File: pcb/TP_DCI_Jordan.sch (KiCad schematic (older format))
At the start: 19 parts, among them J1 MICRO, J2 Display, SW1 SW_DIP_x03, U1 PCF8574

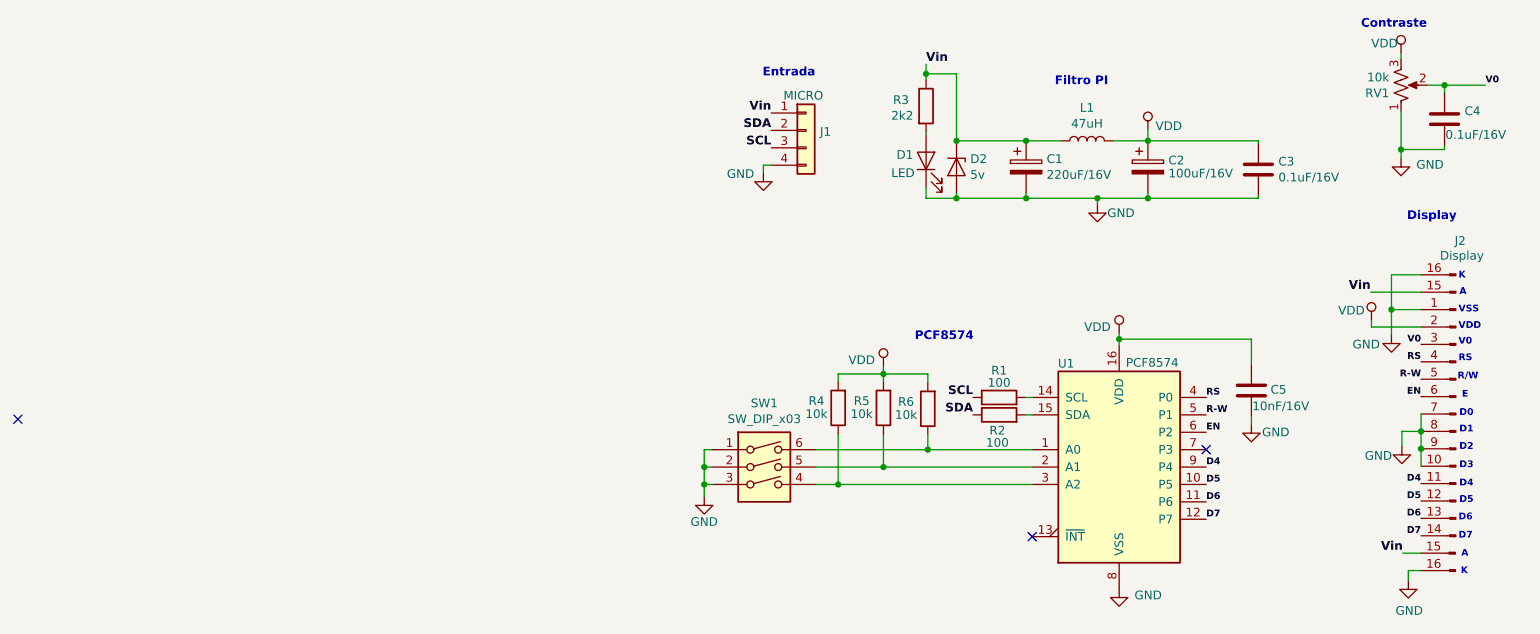
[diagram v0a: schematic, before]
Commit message: mejora de esquemático
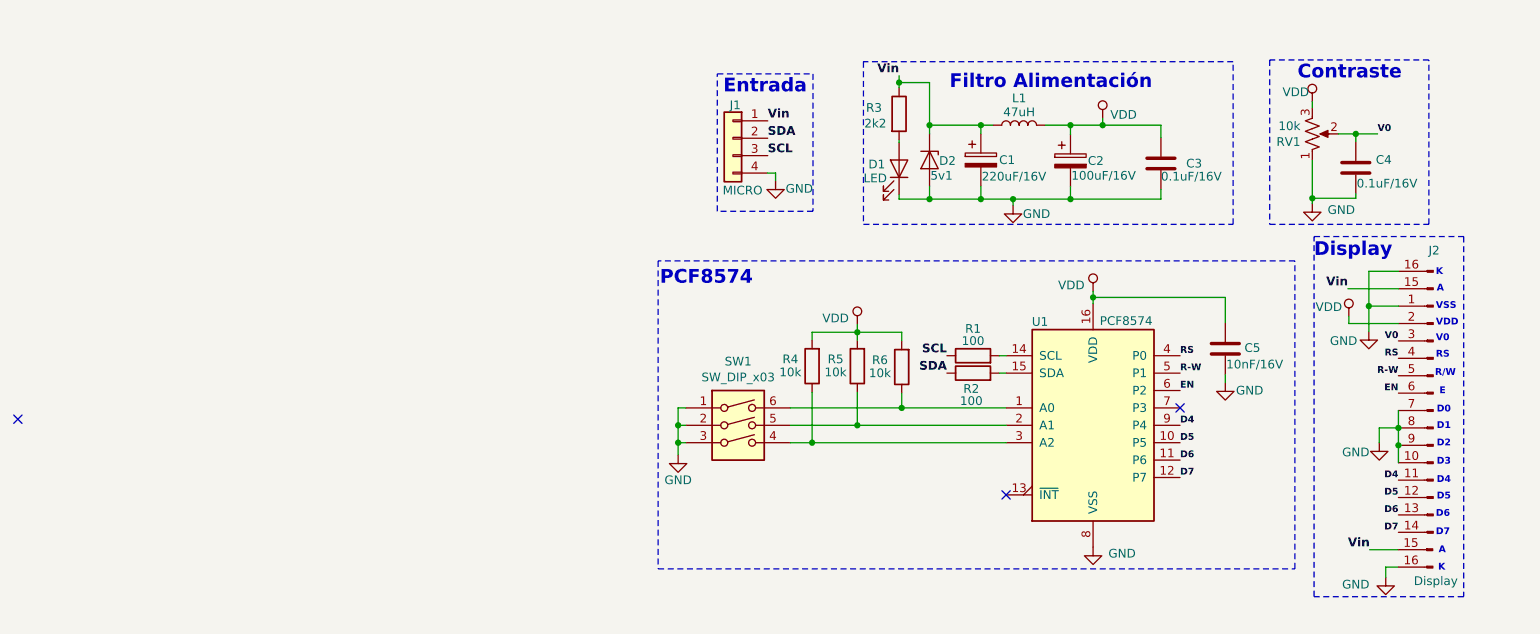
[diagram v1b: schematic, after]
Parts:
- C3, C4, C5: footprint miCapacitor_THT:Lenteja_Ceramica -> Capacitor_SMD:C_0805_2012Metric
- D2: value 5v -> 5v1
- R1, R2, R3, R4, R5, R6: footprint Resistor_THT:R_Axial_DIN0207_L6.3mm_D2.5mm_P7.62mm_Horizontal -> Resistor_SMD:R_0805_2012Metric
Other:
- note added: "Filtro Alimentación"
- note removed: "Filtro PI"
- moved on the sheet: C1, C2, C3, C4, C5, D1, D2, J1, J2, L1, R1, R2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
